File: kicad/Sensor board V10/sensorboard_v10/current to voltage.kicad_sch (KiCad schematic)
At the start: 12 parts, among them J4 Conn_01x02, J5 Conn_01x02, J8 Conn_01x02, J9 Conn_01x02, U6 LM324

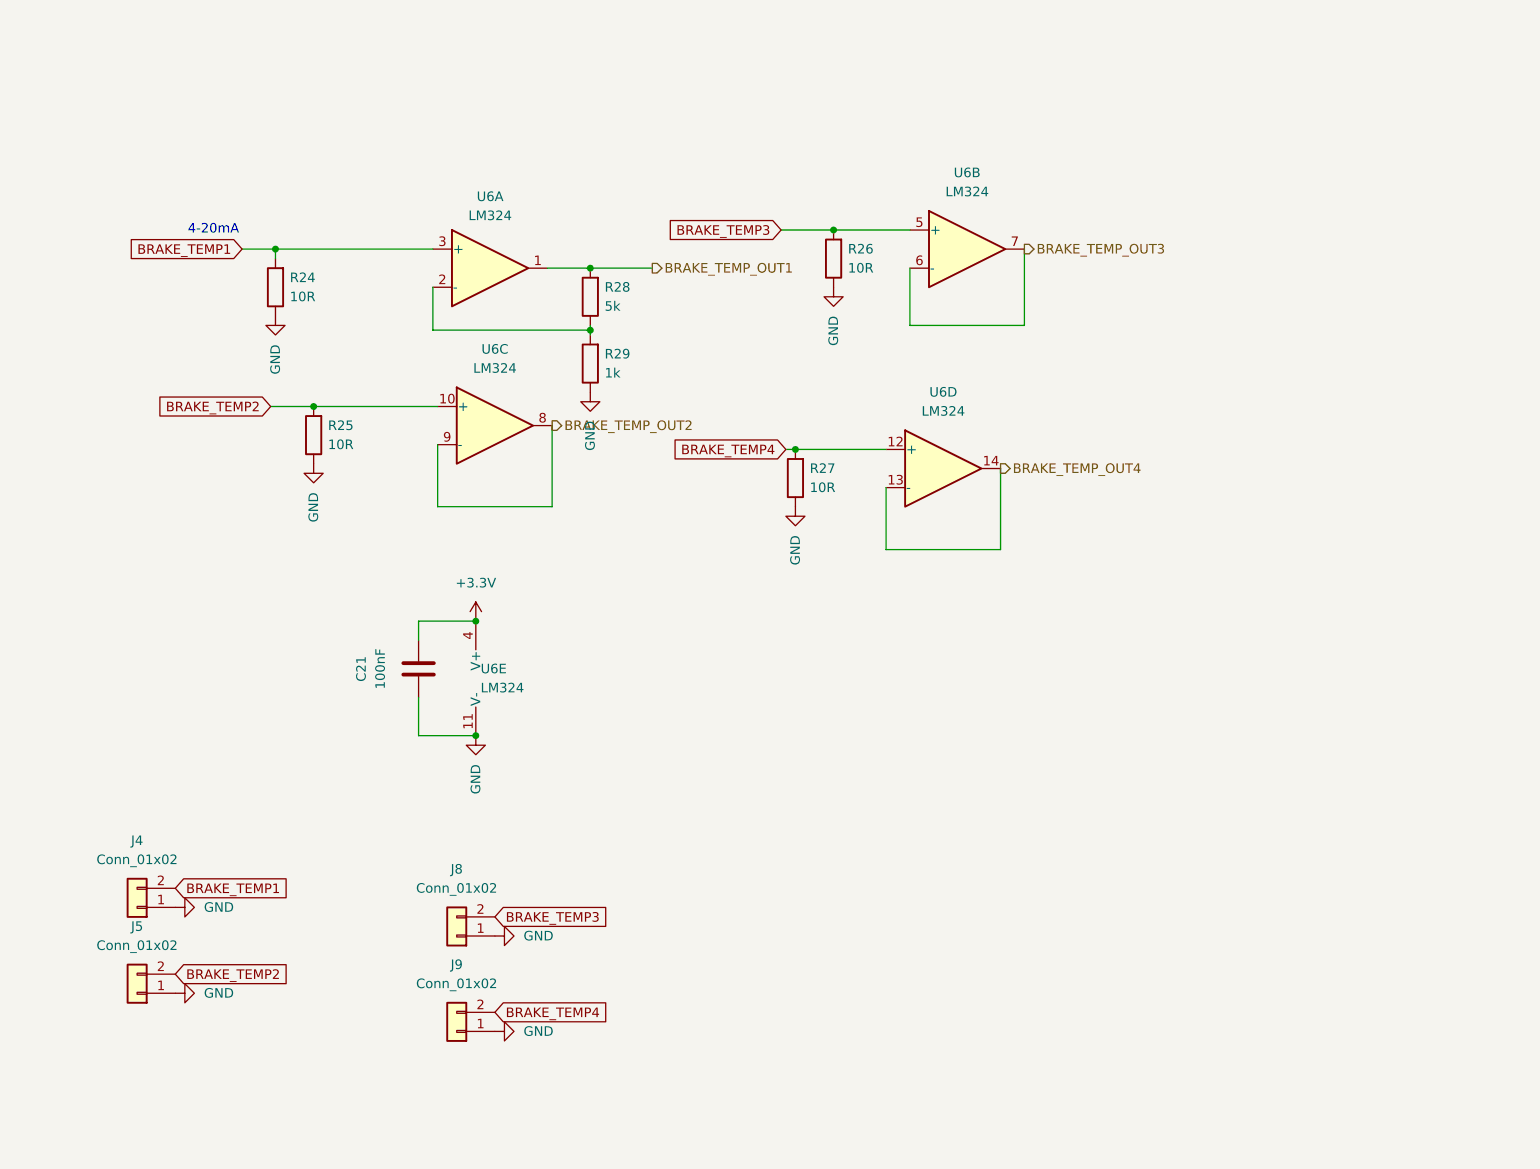
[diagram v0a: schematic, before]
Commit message: Sensor Board V10 schematics
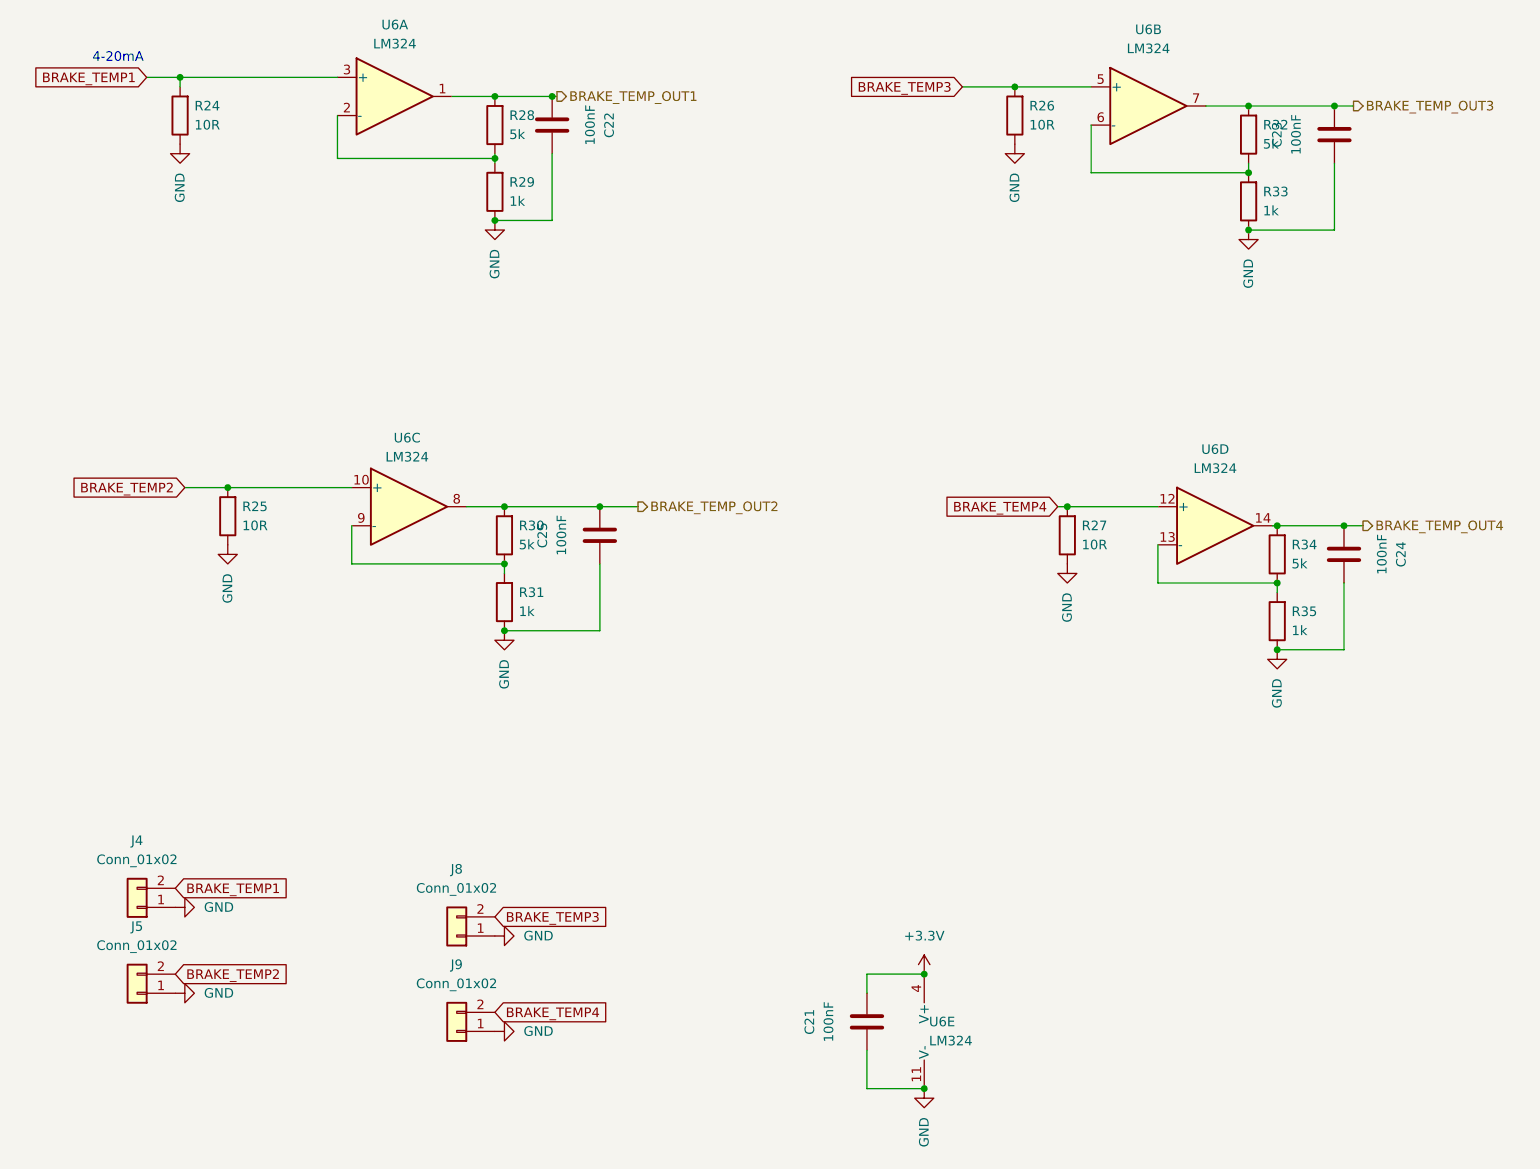
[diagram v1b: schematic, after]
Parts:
- added C22, C23, C24, C25: 100nF, RMC_Capacitor:C_0805_2012Metric_Pad1.18x1.45mm_HandSolder_L, symbol Device:C
- added R30, R32, R34: 5k, RMC_Resistor:R_0805_2012Metric_Pad1.20x1.40mm_HandSolder_L, symbol Device:R
- added R31, R33, R35: 1k, RMC_Resistor:R_0805_2012Metric_Pad1.20x1.40mm_HandSolder_L, symbol Device:R
- R24, R25, R26, R27: footprint RMC_Resistor:R_0805_2012Metric_Pad1.20x1.40mm_HandSolder_L -> RMC_Resistor:R_1206_3216Metric_Pad1.30x1.75mm_HandSolder_RMC
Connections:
- net BRAKE_TEMP_OUT1: now also C22.1
- net BRAKE_TEMP_OUT2: now also C25.1, R30.2; no longer U6.9 (-)
- net BRAKE_TEMP_OUT3: now also C23.1, R32.2; no longer U6.6 (-)
- net BRAKE_TEMP_OUT4: now also C24.1, R34.2; no longer U6.13 (-)
- net GND: now also C22.2, C23.2, C24.2, C25.2, R31.1, R33.1, R35.1
- new net: R30.1, R31.2, U6.9 (-)
- new net: R34.1, R35.2, U6.13 (-)
- new net: R32.1, R33.2, U6.6 (-)
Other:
- moved on the sheet: C21, R24, R25, R26, R27, R28, R29, U6A, U6B, U6C, U6D, U6E
